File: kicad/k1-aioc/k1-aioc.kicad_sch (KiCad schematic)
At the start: 46 parts, among them J1 12401832E402A, J2 Conn_01x07_Male, Q1 BC847BS, U1 MIC5330-SSYML, U2 STM32F373CBTx, Y1 8MHz/20pF

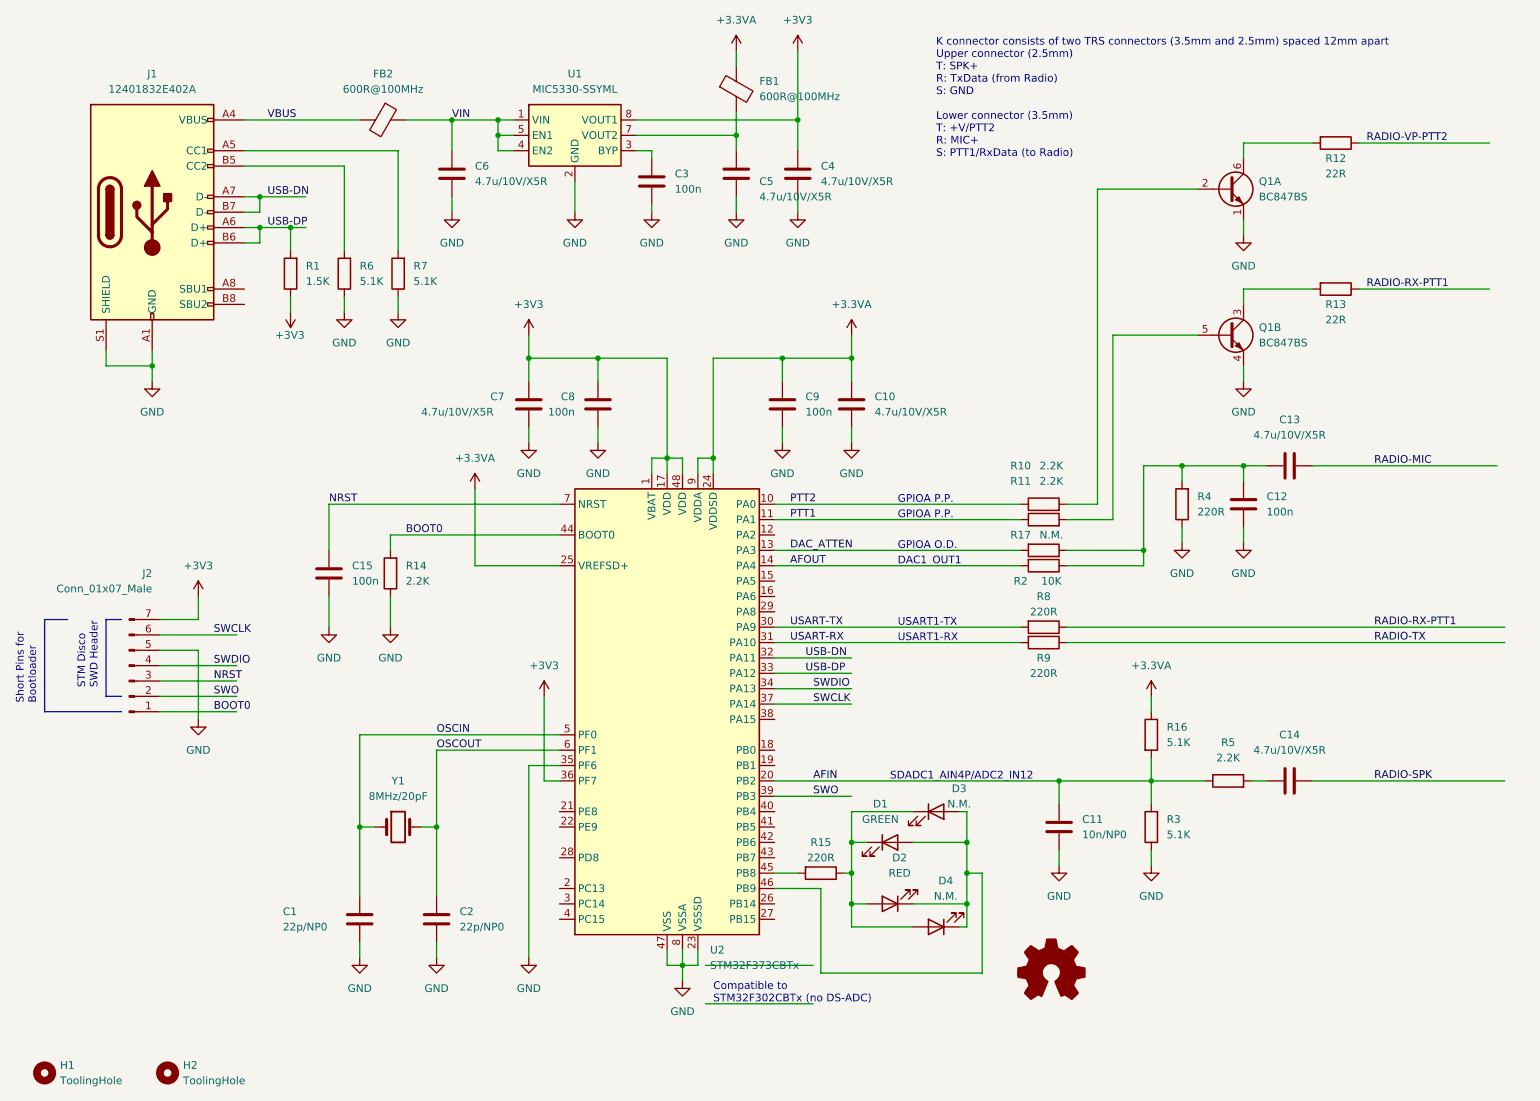
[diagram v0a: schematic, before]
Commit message: Upgraded to latest version
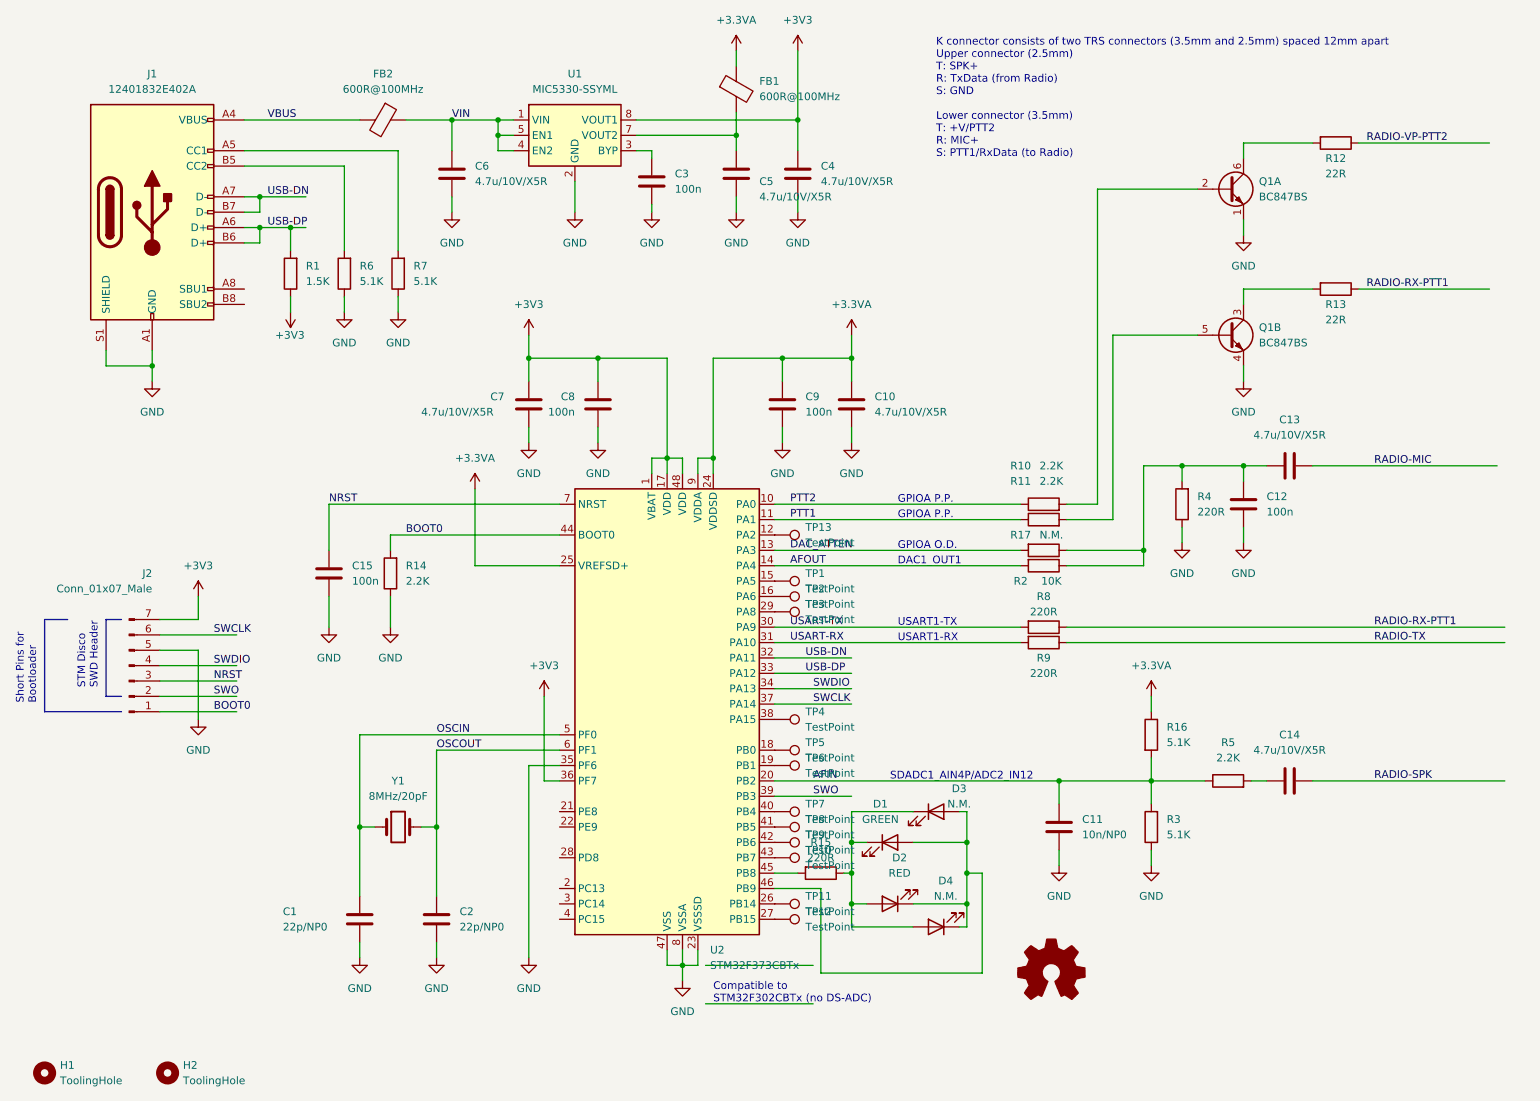
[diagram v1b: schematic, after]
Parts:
- added TP1, TP10, TP11, TP12, TP13, TP2, TP3, TP4, TP5, TP6, TP7, TP8, TP9: TestPoint, TestPoint:TestPoint_Pad_1.0x1.0mm, symbol Connector:TestPoint
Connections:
- net at U2.12 (PA2): now also TP13.1
- net at U2.15 (PA5): now also TP1.1
- net at U2.16 (PA6): now also TP2.1
- net at U2.18 (PB0): now also TP5.1
- net at U2.19 (PB1): now also TP6.1
- net at U2.26 (PB14): now also TP11.1
- net at U2.27 (PB15): now also TP12.1
- net at U2.29 (PA8): now also TP3.1
- net at U2.38 (PA15): now also TP4.1
- net at U2.40 (PB4): now also TP7.1
- net at U2.41 (PB5): now also TP8.1
- net at U2.42 (PB6): now also TP9.1
- net at U2.43 (PB7): now also TP10.1
